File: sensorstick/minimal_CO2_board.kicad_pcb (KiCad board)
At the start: 2 copper layers, 80 x 28 mm, 5 parts, among them J1 USB_A, U1 ESP32-C3_SUPERMINI

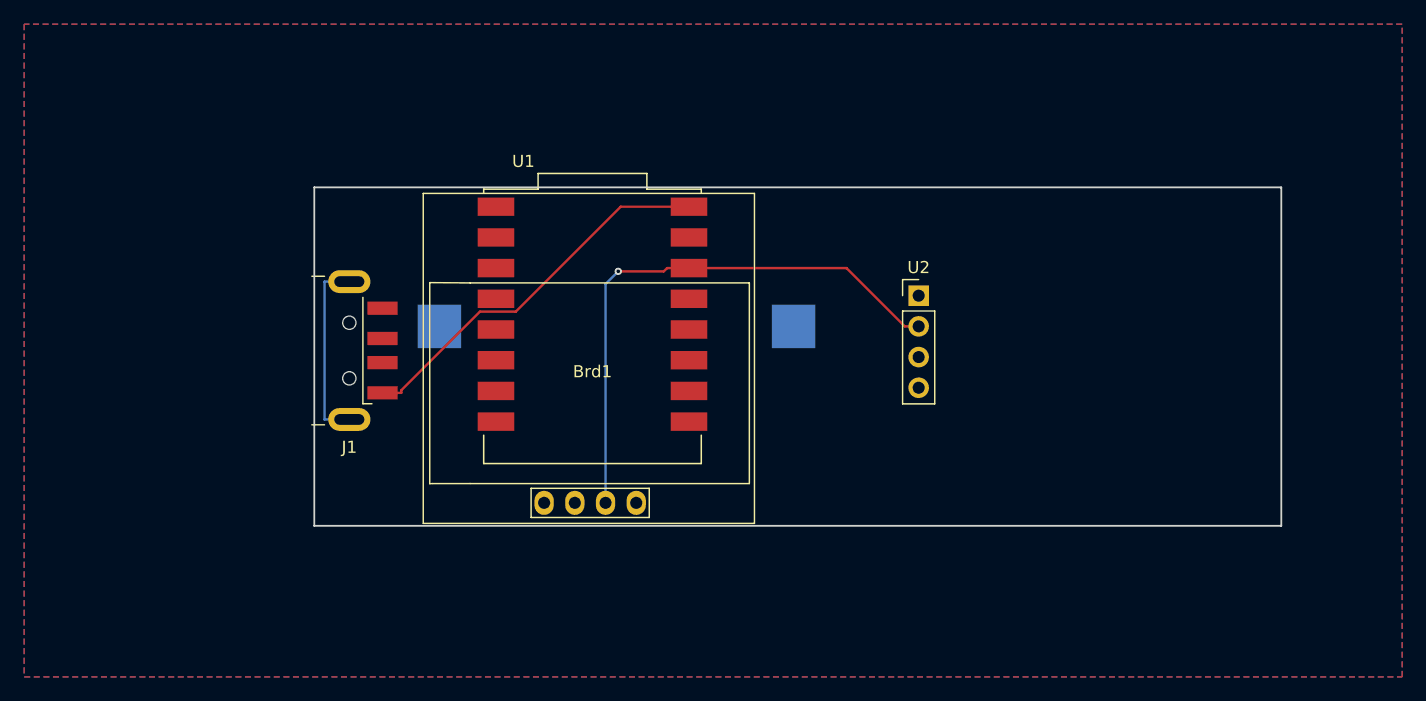
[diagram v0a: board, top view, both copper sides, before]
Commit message: add stuff
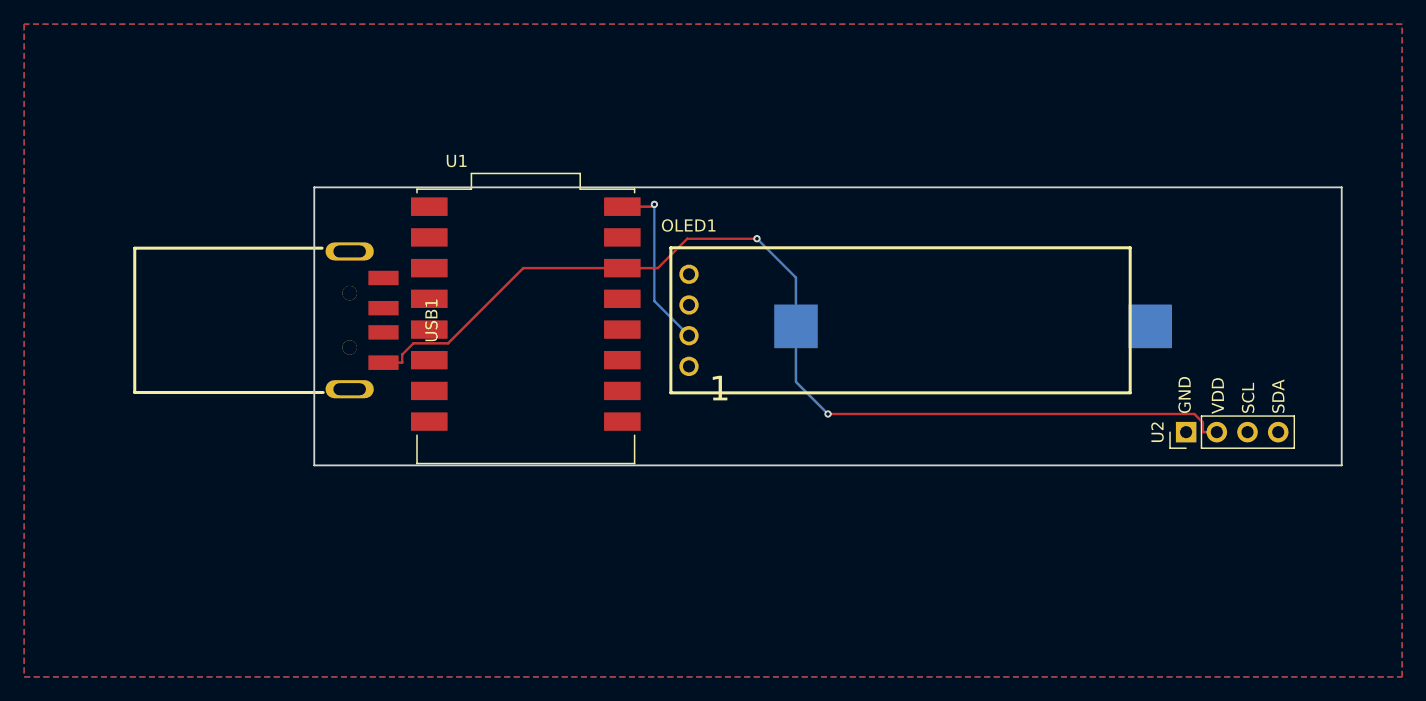
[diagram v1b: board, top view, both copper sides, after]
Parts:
- removed Brd1: SSD1306, CustomLibrary:128x64OLED
- removed J1: USB_A, Connector_USB:USB_A_CNCTech_1001-011-01101_Horizontal
- added OLED1: HS91L02W2C01, CustomLibrary:OLED-TH_L38.0-W12.0_HS91L02W2C01, F.Cu at (91.0, 98.5)
- added USB1: U217-04XN-XXR84, CustomLibrary:USB-A-SMD_U217-041N-4BV81, F.Cu at (64.3, 98.5)
- moved BT1 29.5 mm to (114.5, 99.0)
- moved U2 24.8 mm to (132.1, 107.8), turned to 90 degrees
- moved U1 5.52 mm to (77.5, 99.0)
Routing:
- net +3.3V: track 46.5 -> 85.7 mm, vias 1 -> 2
- net +5V: track 31.9 -> 14.8 mm, vias 0 -> 1
- net unconnected-(J1-Shield-Pad5): track 15.5 -> 0.00 mm
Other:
- board size 80 x 28 mm -> 85 x 23 mm
